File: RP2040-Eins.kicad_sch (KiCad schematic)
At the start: 37 parts, among them J5 CONN_R3, J6 USB_B_Micro, J7 CONN_JTAG, Q1 AO3400A, U1 W25Q128JVS, U2 RP2040, U3 AMS1117-5.0, U4 W25Q128JVEIQ, U5 AMS1117-3.3, Y1 12MHz

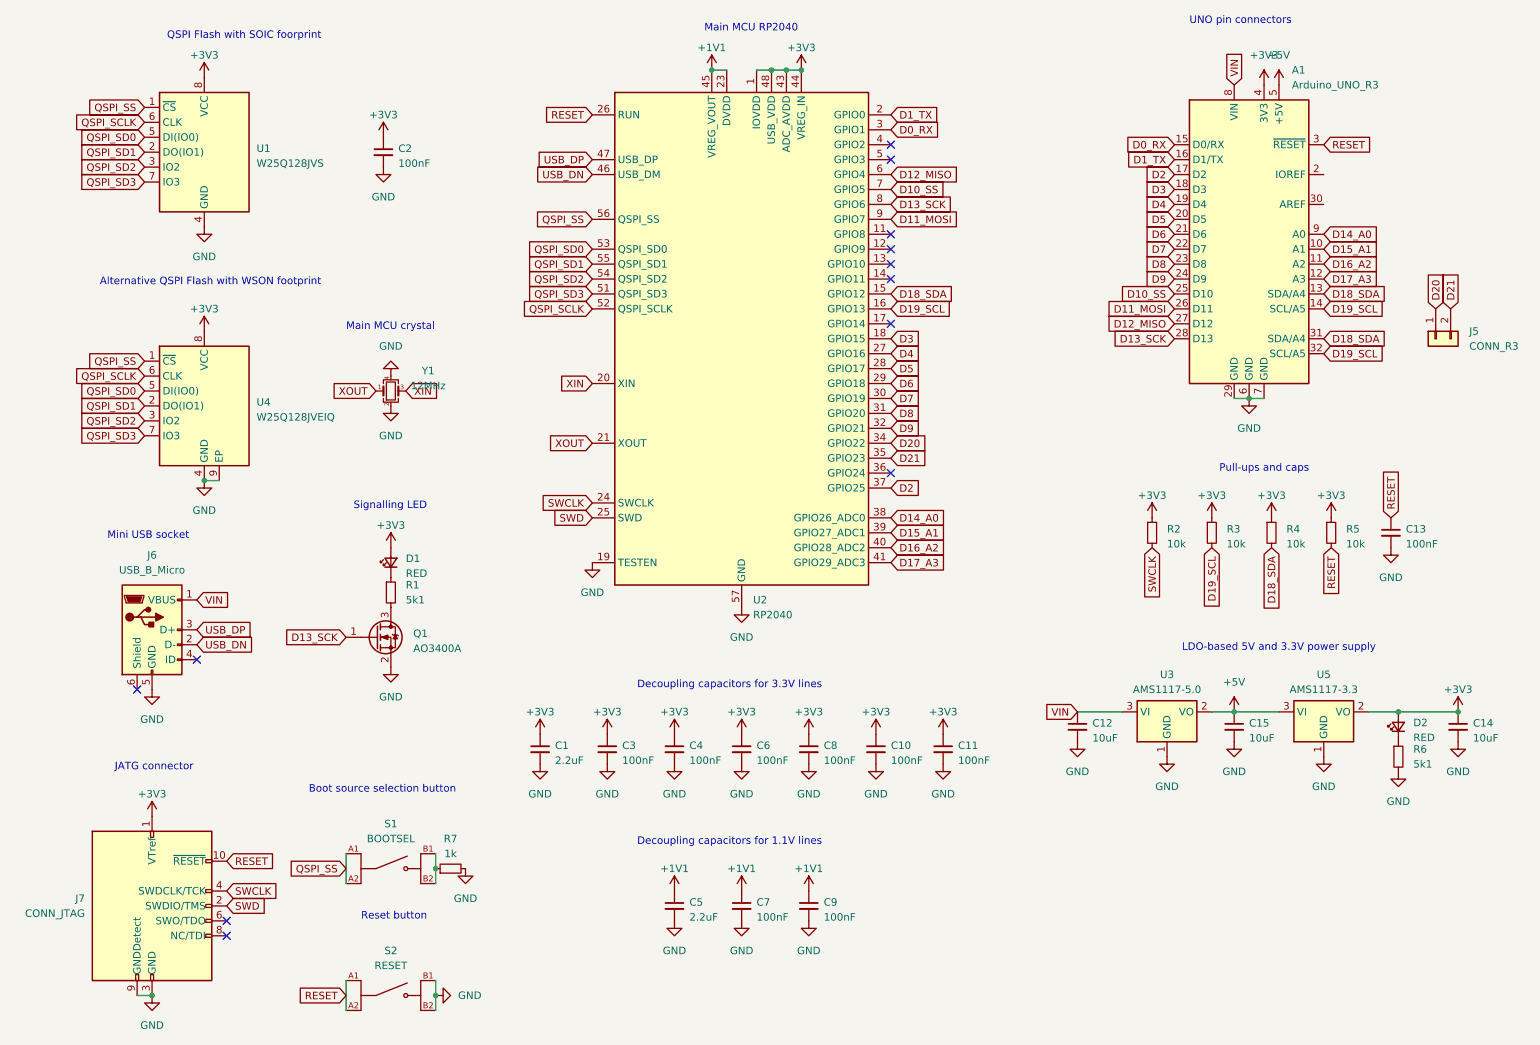
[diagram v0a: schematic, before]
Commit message: Added few components
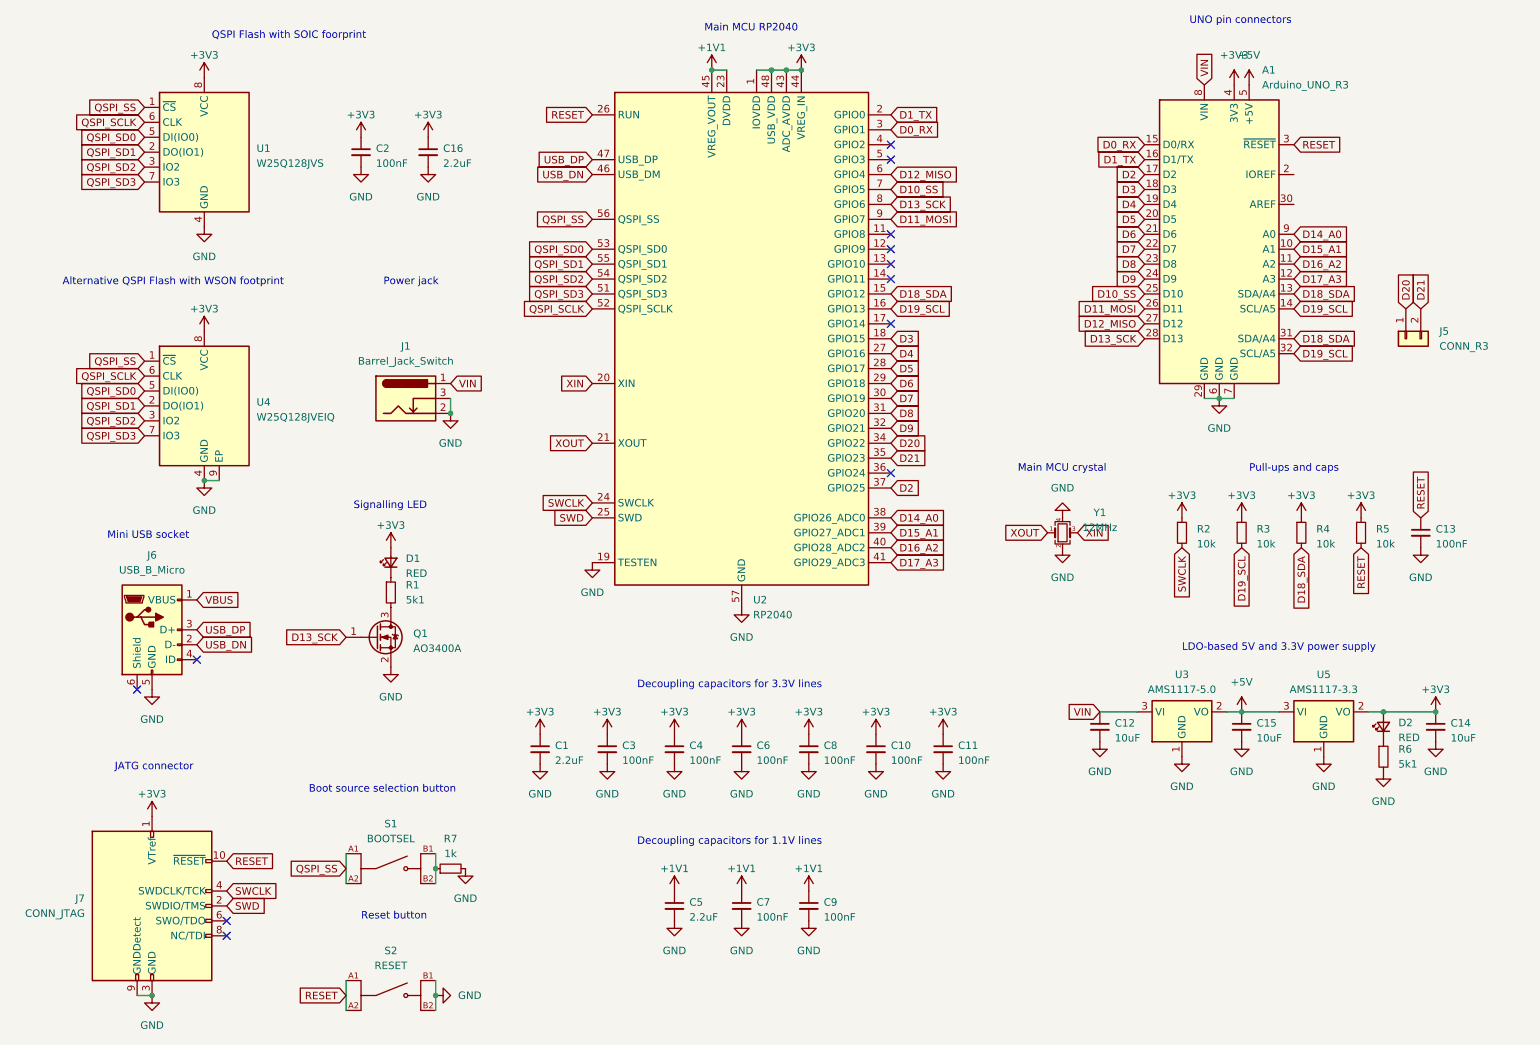
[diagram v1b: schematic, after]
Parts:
- added C16: 2.2uF, Capacitor_SMD:C_0603_1608Metric, symbol Device:C_Small
- added J1: Barrel_Jack_Switch, Connector_BarrelJack:BarrelJack_Horizontal, symbol Connector:Barrel_Jack_Switch
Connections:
- net +3V3: now also C16.1
- net GND: now also C16.2, J1.2, J1.3
- net VIN: now also J1.1; no longer J6.1 (VBUS)
- new net VBUS: J6.1 (VBUS)
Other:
- note added: "Power jack"
- moved on the sheet: A1, C12, C13, C14, C15, C2, D2, J5, R2, R3, R4, R5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
